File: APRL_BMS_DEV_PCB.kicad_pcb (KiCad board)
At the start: 4 copper layers, 73 parts, among them J1 Conn_01x04_Pin, J3 Conn_01x02_Pin, J4 Conn_01x08_Pin, J5 Conn_01x01_Pin, Q1 Q_NPN, SW1 SW_SPDT, U1 BQ756506-Q1, U2 STM32F446RCTx, U3 ISO7741DWR, Y1 20MHz

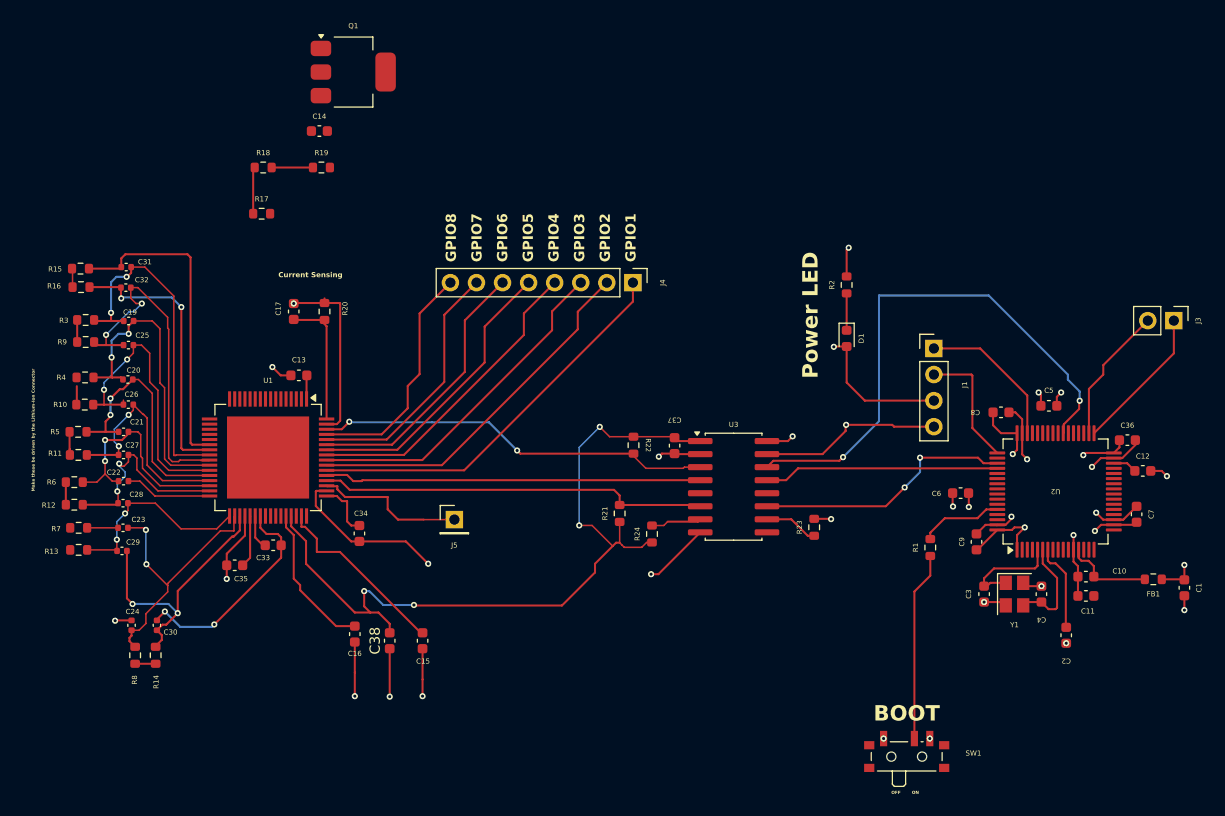
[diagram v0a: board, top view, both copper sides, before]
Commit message: Finished initial trace.
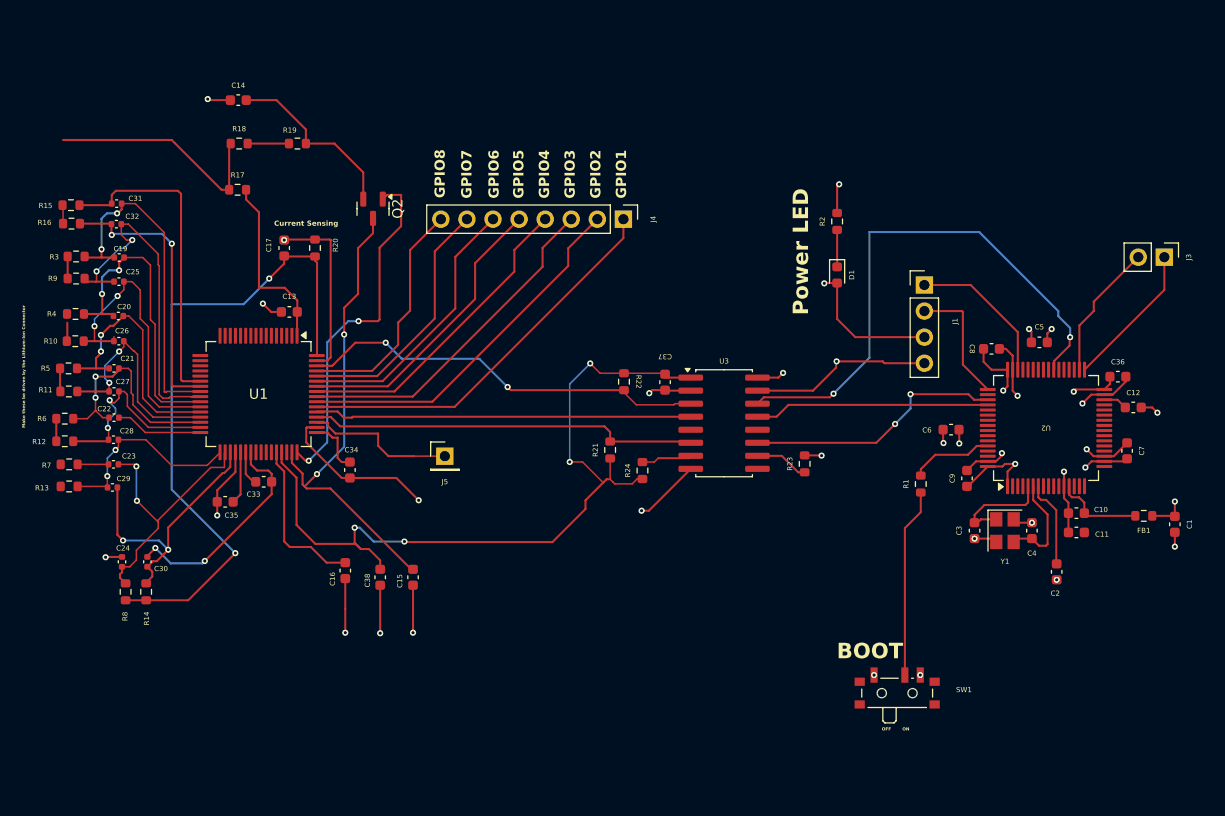
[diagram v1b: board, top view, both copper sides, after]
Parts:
- removed Q1: Q_NPN, Package_TO_SOT_SMD:SOT-223
- added Q2: NPN, Package_TO_SOT_SMD:SOT-23, F.Cu at (121.5, 72.0)
- U1: footprint Package_QFP:HTQFP-64-1EP_10x10mm_P0.5mm_EP8x8mm -> Package_QFP:LQFP-64_10x10mm_P0.5mm
- moved C14 8.46 mm to (108.4, 61.4)
- moved C1 6.25 mm to (199.6, 102.7)
- moved C15 6.25 mm to (125.4, 107.8)
- moved C29 6.25 mm to (96.1, 99.1)
- moved C30 6.25 mm to (99.5, 106.3)
- moved C38 6.25 mm to (122.2, 107.8)
- moved C6 6.25 mm to (177.8, 93.5)
- moved C9 6.25 mm to (179.4, 98.2)
- moved J1 6.25 mm to (175.2, 79.4)
- moved J4 6.25 mm to (145.9, 73.0)
- moved J5 6.25 mm to (128.5, 96.0)
- moved R1 6.25 mm to (174.9, 98.8)
- moved R10 6.25 mm to (92.5, 84.8)
- moved R11 6.25 mm to (91.9, 89.8)
- moved R13 6.25 mm to (91.9, 99.0)
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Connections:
- net Net-(C14-Pad2) renamed /Collector
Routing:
- net /CELL_0: track 14.8 -> 65.5 mm, vias 0 -> 2
- net /NPNB: track 0.00 -> 34.8 mm, vias 0 -> 2
- net /LDOIN: track 17.9 -> 46.6 mm, vias 0 -> 2
- net /CELL_6: track 6.38 -> 24.6 mm
- net /Collector: track 0.00 -> 17.7 mm
- net /BAT: track 2.31 -> 17.7 mm
- net GND: track 149.2 -> 151.0 mm, vias 27 -> 28
- net /CVDD: track 78.0 -> 79.4 mm
- net /NFAULT: track 38.8 -> 40.0 mm
- net /NEG5V: track 14.6 -> 15.8 mm
